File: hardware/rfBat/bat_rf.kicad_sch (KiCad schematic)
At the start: 90 parts, among them J1 USB_C_Receptacle_PowerOnly_6P, J2 Conn_01x01_Pin, J3 Conn_01x06, J4 Conn_01x03, J5 Conn_01x01_Pin, Q1 Q_PMOS_GDS, Q2 AllPower__AP2300, Q5 AllPower__AP2300, SW2 3*4*2.5MM_贴片4脚, SW3 TS-1199A-B-B, U1 ESP32-C3-WROOM-02-N4, U2 IP2325_5M_WHJC, U4 AMS1117, U5 MLT-8530-5V, U7 XC6220B331MR

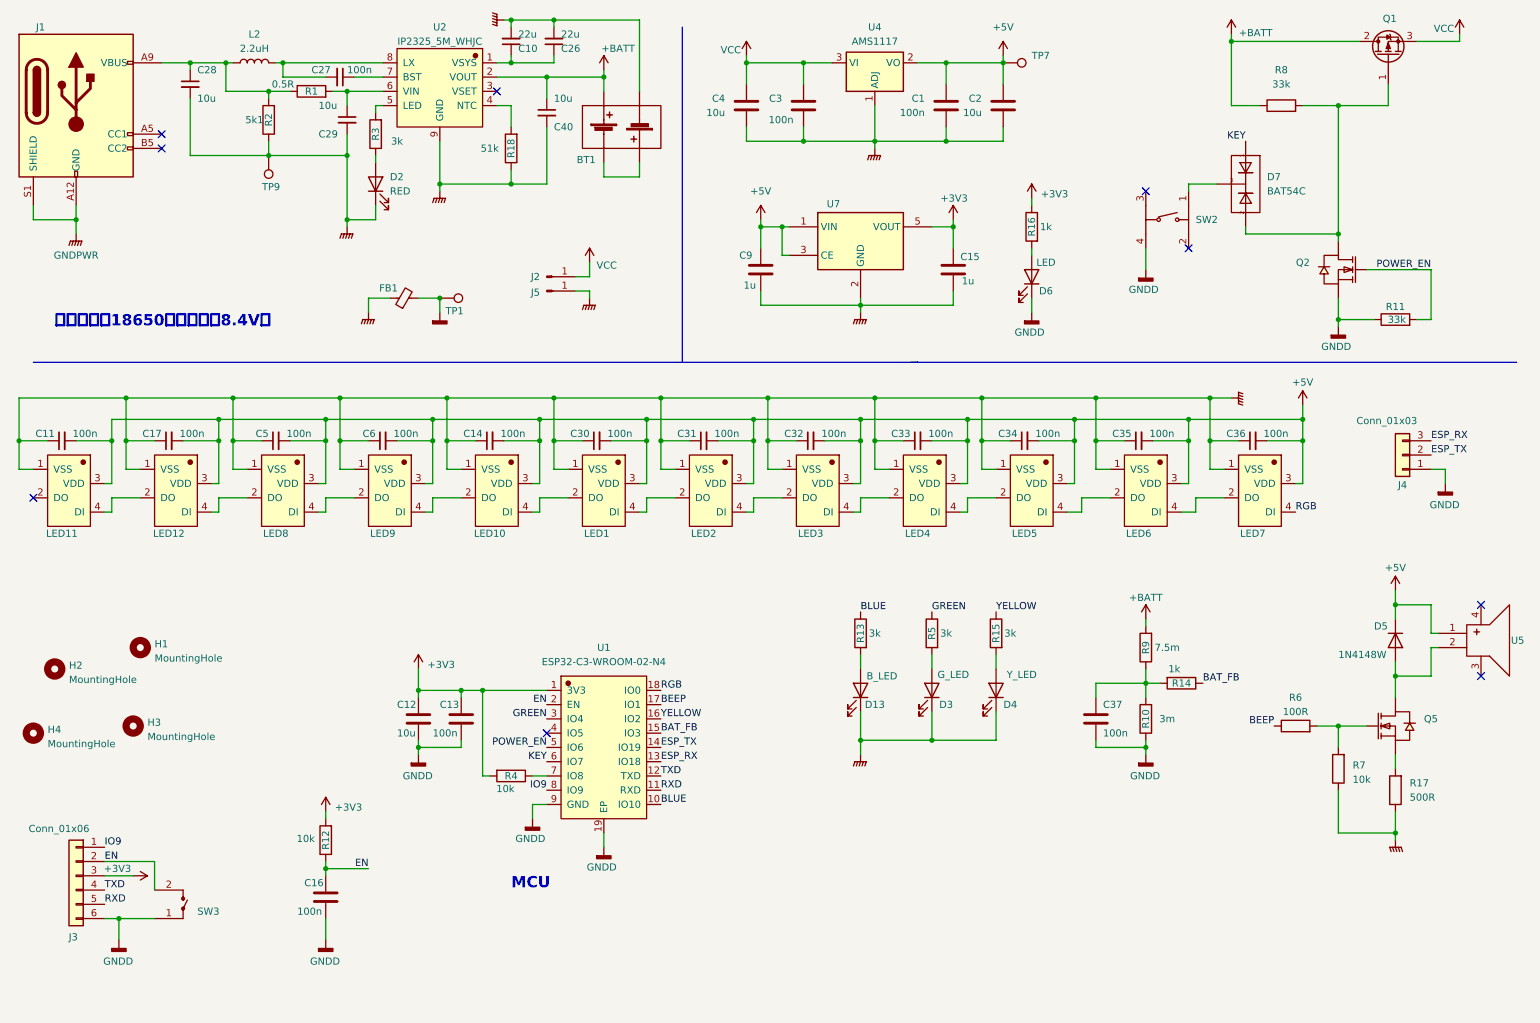
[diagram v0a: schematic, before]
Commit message: update pcn
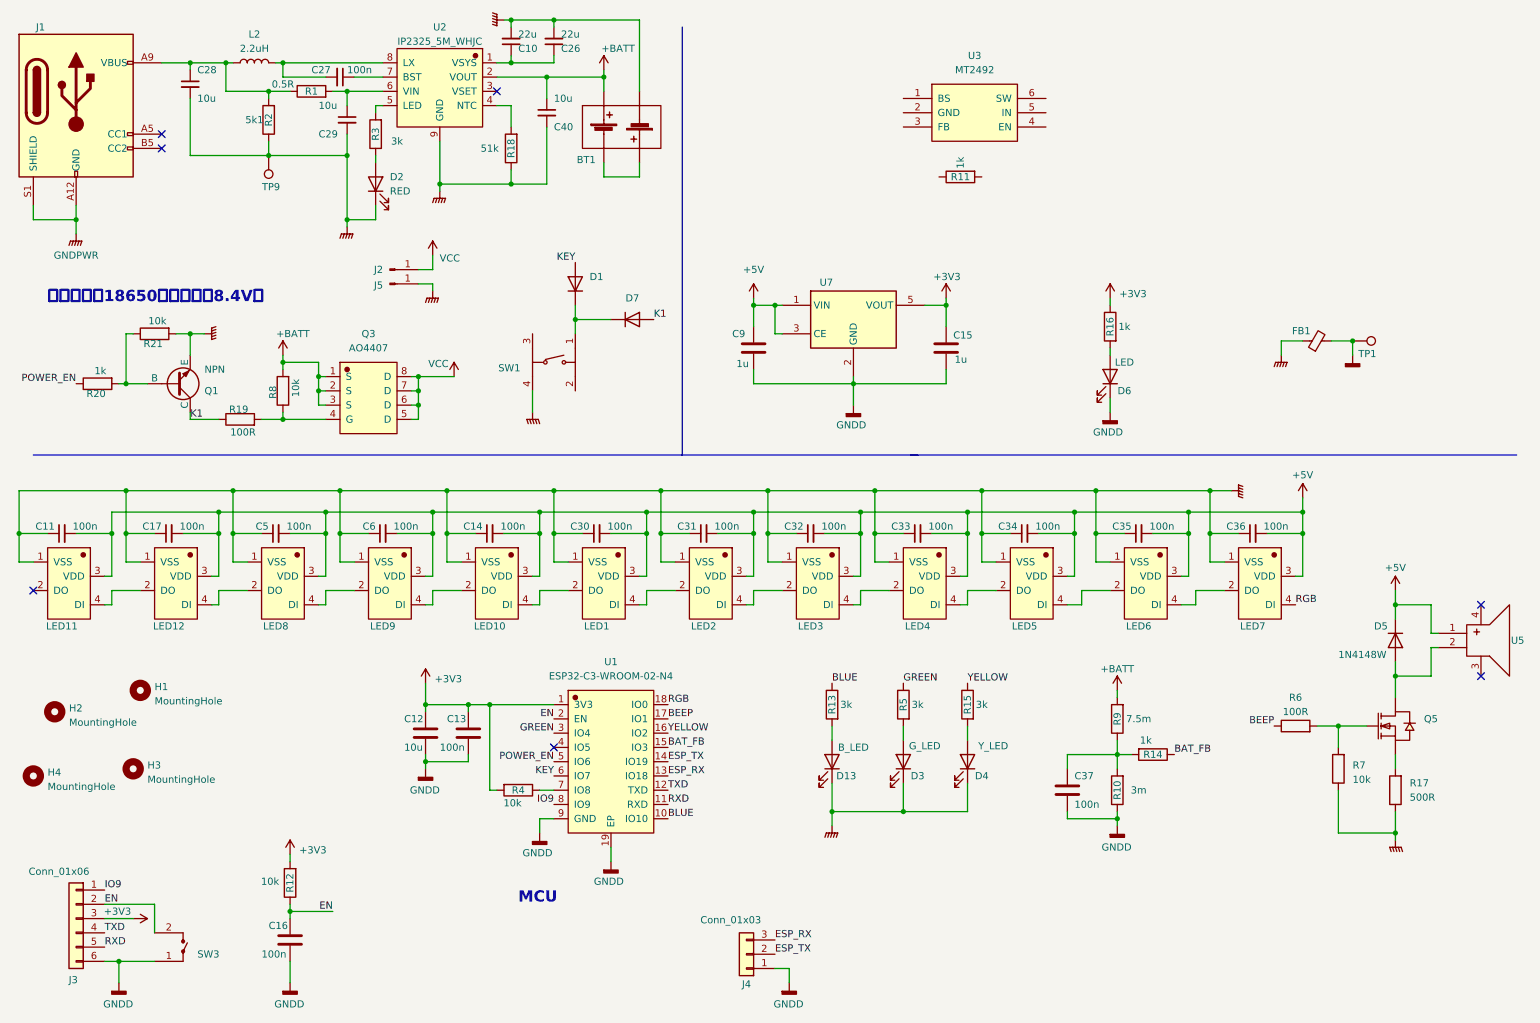
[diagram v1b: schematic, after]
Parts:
- removed C1, C3: 100n, Capacitor_SMD:C_0603_1608Metric_Pad1.08x0.95mm_HandSolder, symbol Device:C
- removed C2, C4: 10u, Capacitor_SMD:C_0805_2012Metric_Pad1.18x1.45mm_HandSolder, symbol Device:C
- removed D7: BAT54C, bat_rf:BAT54C, symbol bat_rf:BAT54C
- removed Q1: Q_PMOS_GDS, Package_TO_SOT_SMD:TO-252-2, symbol Device:Q_PMOS_GDS
- removed Q2: AllPower__AP2300, bat_rf:SOT-23, symbol bat_rf:AllPower__AP2300
- removed SW2: 3*4*2.5MM_贴片4脚, bat_rf:SW-SMD_4P-L4.2-W3.3-P2.15-LS5.1, symbol bat_rf:3*4*2.5MM_贴片4脚
- removed TP7: TestPoint, TestPoint:TestPoint_Pad_D1.0mm, symbol Connector:TestPoint
- removed U4: AMS1117, Package_TO_SOT_SMD:SOT-89-3_Handsoldering, symbol Regulator_Linear:AMS1117
- added D1, D7: 1N4148W, Diode_SMD:D_SOD-123, symbol Diode:1N4148W
- added Q1: NPN, symbol Simulation_SPICE:NPN
- added Q3: AO4407, bat_rf:SOP-8_L5.0-W4.0-P1.27-LS6.0-BL, symbol bat_rf:AO4407
- added R19: 100R, Resistor_SMD:R_0603_1608Metric_Pad0.98x0.95mm_HandSolder, symbol Device:R
- added R20: 1k, Resistor_SMD:R_0603_1608Metric_Pad0.98x0.95mm_HandSolder, symbol Device:R
- added R21: 10k, Resistor_SMD:R_0603_1608Metric_Pad0.98x0.95mm_HandSolder, symbol Device:R
- added SW1: 3*4*2.5MM_贴片4脚, bat_rf:SW-SMD_4P-L4.2-W3.3-P2.15-LS5.1, symbol bat_rf:3*4*2.5MM_贴片4脚
- added U3: MT2492, bat_rf:SOT-23-6_L2.9-W1.6-P0.95-LS2.8-BL, symbol bat_rf:MT2492
- R11: value 33k -> 1k
- R8: value 33k -> 10k
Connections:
- net +BATT: now also R8.2, Q3.1 (S), Q3.2 (S), Q3.3 (S); no longer R8.1
- net GNDD: now also C15.2, C9.2, U7.2 (GND); no longer R11.1
- net GNDPWR: now also Q1.3 (E), R21.2, SW1.4; no longer C15.2, C9.2, U7.2 (GND)
- net KEY: now also D1.2 (A)
- net POWER_EN: now also R20.1; no longer R11.2
- net VCC: now also Q3.5 (D), Q3.6 (D), Q3.7 (D), Q3.8 (D)
- new net: Q1.2 (B), R20.2, R21.1
- new net: Q3.4 (G), R19.2, R8.1
- new net: D1.1 (K), D7.1 (K), SW1.1
- new net K1: D7.2 (A), Q1.1 (C), R19.1
- no-connect marks 9 -> 7
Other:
- moved on the sheet: C11, C12, C13, C14, C15, C16, C17, C30, C31, C32, C33, C34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
